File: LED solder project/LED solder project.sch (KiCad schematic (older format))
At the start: 11 parts, among them Q1 PN2222A, SW1 SW_SPST

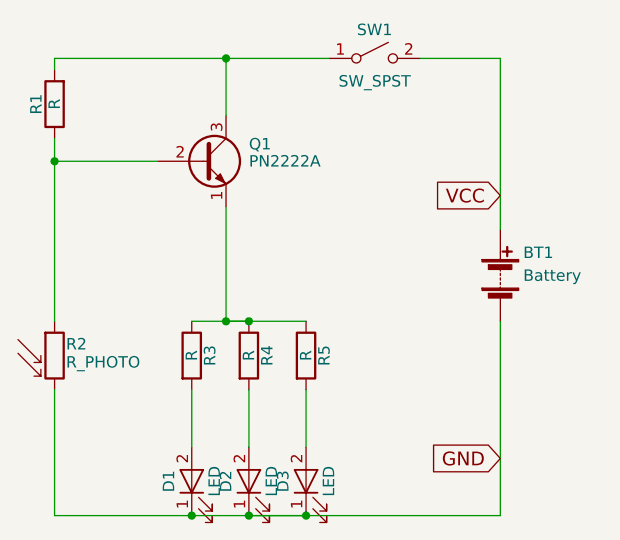
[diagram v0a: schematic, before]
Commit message: added many
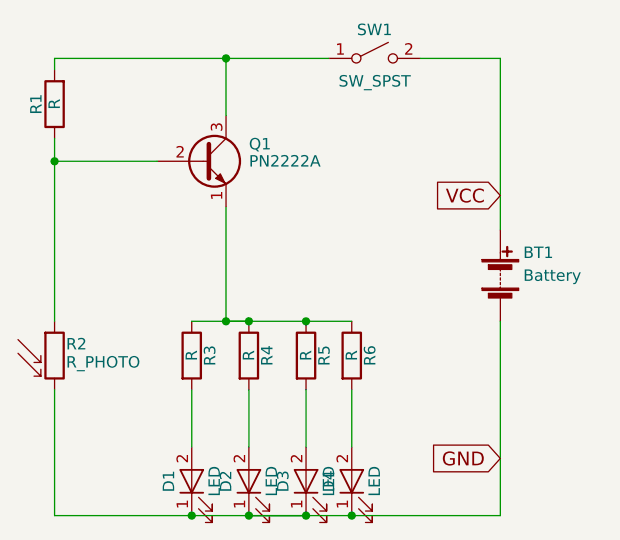
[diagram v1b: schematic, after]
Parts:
- added D4: LED, rocketlib:LED, symbol LED
- added R6: R, rocketlib:resistor, symbol R
- BT1: footprint Pin_Headers:Pin_Header_Straight_2x01_Pitch2.54mm -> rocketlib:Battery
- D1, D2, D3: footprint LEDs:LED_D5.0mm -> rocketlib:LED
- Q1: footprint TO_SOT_Packages_THT:TO-92_Molded_Wide -> rocketlib:transistor
- R1, R3, R4, R5: footprint Resistors_THT:R_Axial_DIN0207_L6.3mm_D2.5mm_P7.62mm_Horizontal -> rocketlib:resistor
- R2: footprint Resistors_THT:R_Axial_DIN0414_L11.9mm_D4.5mm_P5.08mm_Vertical -> rocketlib:Photoresistor
- SW1: footprint Buttons_Switches_THT:SW_DIP_x2_W7.62mm_Piano -> rocketlib:Switch
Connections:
- net GND: now also D4.1 (K)
- net at Q1.1 (E), R3.1, R4.1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: now also R6.1
- new net: D4.2 (A), R6.2
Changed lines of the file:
@@
 LIBS:contrib
 LIBS:valves
+LIBS:LED solder project-cache
 EELAYER 25 0
 EELAYER END
@@
 F 0 "R3" V 3430 4150 50  0000 C CNN
 F 1 "R" V 3350 4150 50  0000 C CNN
-F 2 "Resistors_THT:R_Axial_DIN0207_L6.3mm_D2.5mm_P7.62mm_Horizontal" V 3280 4150 50  0001 C CNN
+F 2 "rocketlib:resistor" V 3280 4150 50  0001 C CNN
 F 3 "" H 3350 4150 50  0001 C CNN
 	1    3350 4150
@@
 F 0 "R4" V 3680 4150 50  0000 C CNN
 F 1 "R" V 3600 4150 50  0000 C CNN
-F 2 "Resistors_THT:R_Axial_DIN0207_L6.3mm_D2.5mm_P7.62mm_Horizontal" V 3530 4150 50  0001 C CNN
+F 2 "rocketlib:resistor" V 3530 4150 50  0001 C CNN
 F 3 "" H 3600 4150 50  0001 C CNN
 	1    3600 4150
@@
 F 0 "R5" V 3930 4150 50  0000 C CNN
 F 1 "R" V 3850 4150 50  0000 C CNN
-F 2 "Resistors_THT:R_Axial_DIN0207_L6.3mm_D2.5mm_P7.62mm_Horizontal" V 3780 4150 50  0001 C CNN
+F 2 "rocketlib:resistor" V 3780 4150 50  0001 C CNN
 F 3 "" H 3850 4150 50  0001 C CNN
 	1    3850 4150
@@
 F 0 "R1" V 2830 3050 50  0000 C CNN
 F 1 "R" V 2750 3050 50  0000 C CNN
-F 2 "Resistors_THT:R_Axial_DIN0207_L6.3mm_D2.5mm_P7.62mm_Horizontal" V 2680 3050 50  0001 C CNN
+F 2 "rocketlib:resistor" V 2680 3050 50  0001 C CNN
 F 3 "" H 2750 3050 50  0001 C CNN
 	1    2750 3050
@@
 F 0 "R2" H 2800 4200 50  0000 L CNN
 F 1 "R_PHOTO" H 2800 4150 50  0000 L TNN
-F 2 "Resistors_THT:R_Axial_DIN0414_L11.9mm_D4.5mm_P5.08mm_Vertical" V 2800 3900 50  0001 L CNN
+F 2 "rocketlib:Photoresistor" V 2800 3900 50  0001 L CNN
 F 3 "" H 2750 4100 50  0001 C CNN
 	1    2750 4150
@@
 F 0 "Q1" H 3600 3375 50  0000 L CNN
 F 1 "PN2222A" H 3600 3300 50  0000 L CNN
-F 2 "TO_SOT_Packages_THT:TO-92_Molded_Wide" H 3600 3225 50  0001 L CIN
+F 2 "rocketlib:transistor" H 3600 3225 50  0001 L CIN
 F 3 "" H 3400 3300 50  0001 L CNN
 	1    3400 3300
@@
 F 0 "D1" H 3350 4800 50  0000 C CNN
 F 1 "LED" H 3350 4600 50  0000 C CNN
-F 2 "LEDs:LED_D5.0mm" H 3350 4700 50  0001 C CNN
+F 2 "rocketlib:LED" H 3350 4700 50  0001 C CNN
 F 3 "" H 3350 4700 50  0001 C CNN
 	1    3350 4700
@@
 F 0 "D2" H 3600 4800 50  0000 C CNN
 F 1 "LED" H 3600 4600 50  0000 C CNN
-F 2 "LEDs:LED_D5.0mm" H 3600 4700 50  0001 C CNN
+F 2 "rocketlib:LED" H 3600 4700 50  0001 C CNN
 F 3 "" H 3600 4700 50  0001 C CNN
 	1    3600 4700
@@
 F 0 "D3" H 3850 4800 50  0000 C CNN
 F 1 "LED" H 3850 4600 50  0000 C CNN
-F 2 "LEDs:LED_D5.0mm" H 3850 4700 50  0001 C CNN
+F 2 "rocketlib:LED" H 3850 4700 50  0001 C CNN
 F 3 "" H 3850 4700 50  0001 C CNN
 	1    3850 4700
@@
 F 0 "SW1" H 4150 2975 50  0000 C CNN
 F 1 "SW_SPST" H 4150 2750 50  0000 C CNN
-F 2 "Buttons_Switches_THT:SW_DIP_x2_W7.62mm_Piano" H 4150 2850 50  0001 C CNN
+F 2 "rocketlib:Switch" H 4150 2850 50  0001 C CNN
 F 3 "" H 4150 2850 50  0001 C CNN
 	1    4150 2850
@@
 F 0 "BT1" H 4800 3900 50  0000 L CNN
 F 1 "Battery" H 4800 3800 50  0000 L CNN
-F 2 "Pin_Headers:Pin_Header_Straight_2x01_Pitch2.54mm" V 4700 3860 50  0001 C CNN
+F 2 "rocketlib:Battery" V 4700 3860 50  0001 C CNN
 F 3 "" V 4700 3860 50  0001 C CNN
 	1    4700 3800
@@
 Connection ~ 3500 2850
 Wire Wire Line
-	3350 4000 3850 4000
+	3350 4000 4050 4000
 Wire Wire Line
 	3500 3500 3500 4000
@@
 Connection ~ 3850 4850
 Connection ~ 3600 4850
+$Comp
+L R R6
+U 1 1 5AA815A9
+P 4050 4150
+F 0 "R6" V 4130 4150 50  0000 C CNN
+F 1 "R" V 4050 4150 50  0000 C CNN
+F 2 "rocketlib:resistor" V 3980 4150 50  0001 C CNN
+F 3 "" H 4050 4150 50  0001 C CNN
+	1    4050 4150
+	1    0    0    -1
+$EndComp
+$Comp
+L LED D4
+U 1 1 5AA815AF
+P 4050 4700
+F 0 "D4" H 4050 4800 50  0000 C CNN
+F 1 "LED" H 4050 4600 50  0000 C CNN
+F 2 "rocketlib:LED" H 4050 4700 50  0001 C CNN
+F 3 "" H 4050 4700 50  0001 C CNN
+	1    4050 4700
+	0    -1   -1   0
+$EndComp
+Wire Wire Line
+	4050 4300 4050 4550
+Connection ~ 3850 4000
+Connection ~ 4050 4850
 $EndSCHEMATC
